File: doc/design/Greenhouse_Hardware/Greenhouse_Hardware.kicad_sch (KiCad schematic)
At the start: 4 parts, among them J1 M5Stack Watering Unit U101, J2 SSD1306 OLED Module, J3 DHT11 module, U1 ESP32-DevKitC

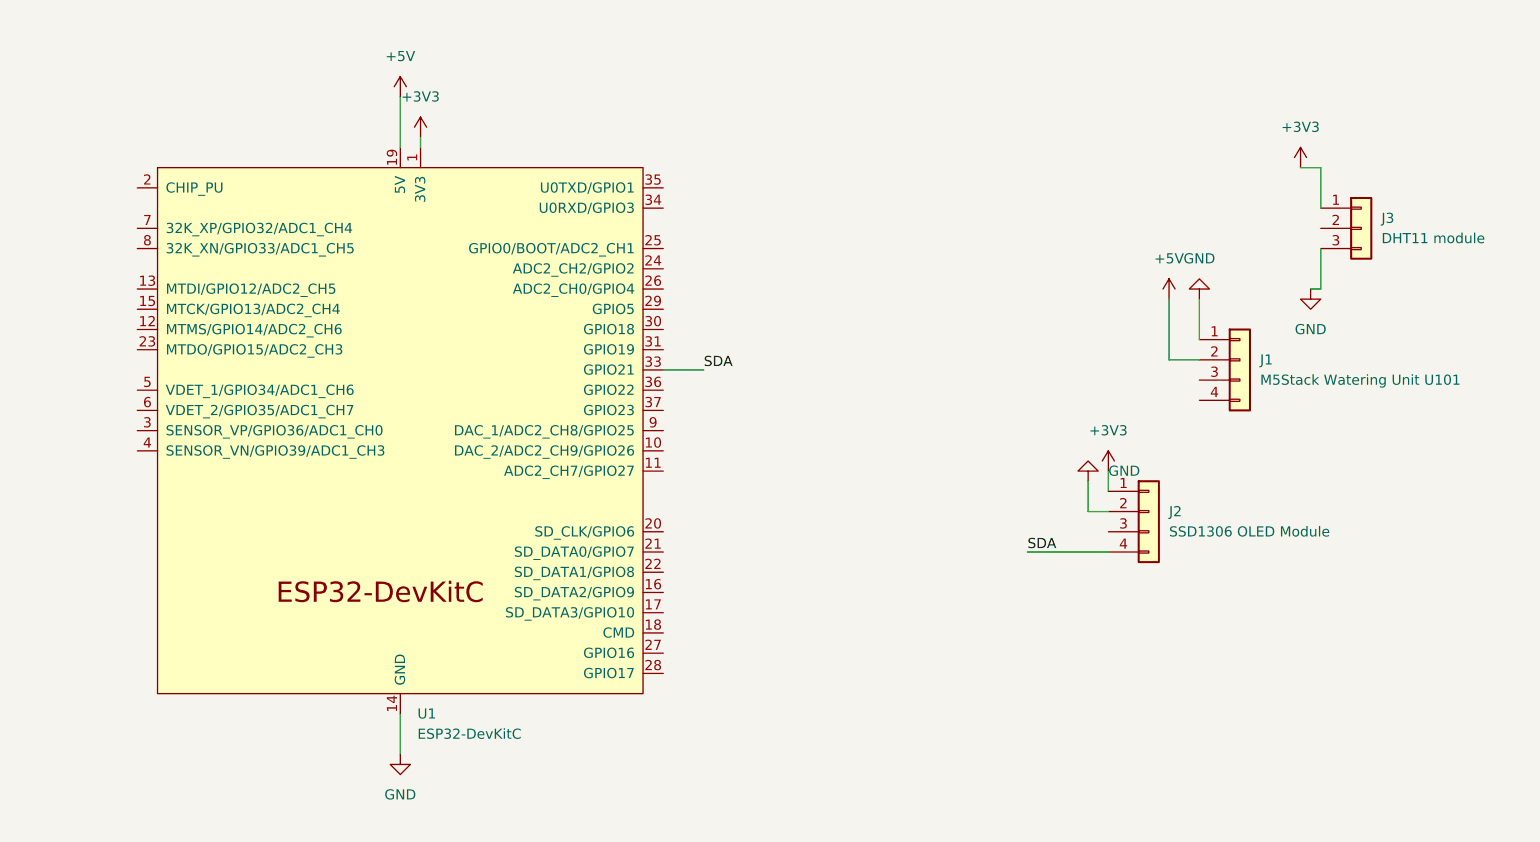
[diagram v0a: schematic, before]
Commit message: WiFi functionallity and sensor reading, validation, data display
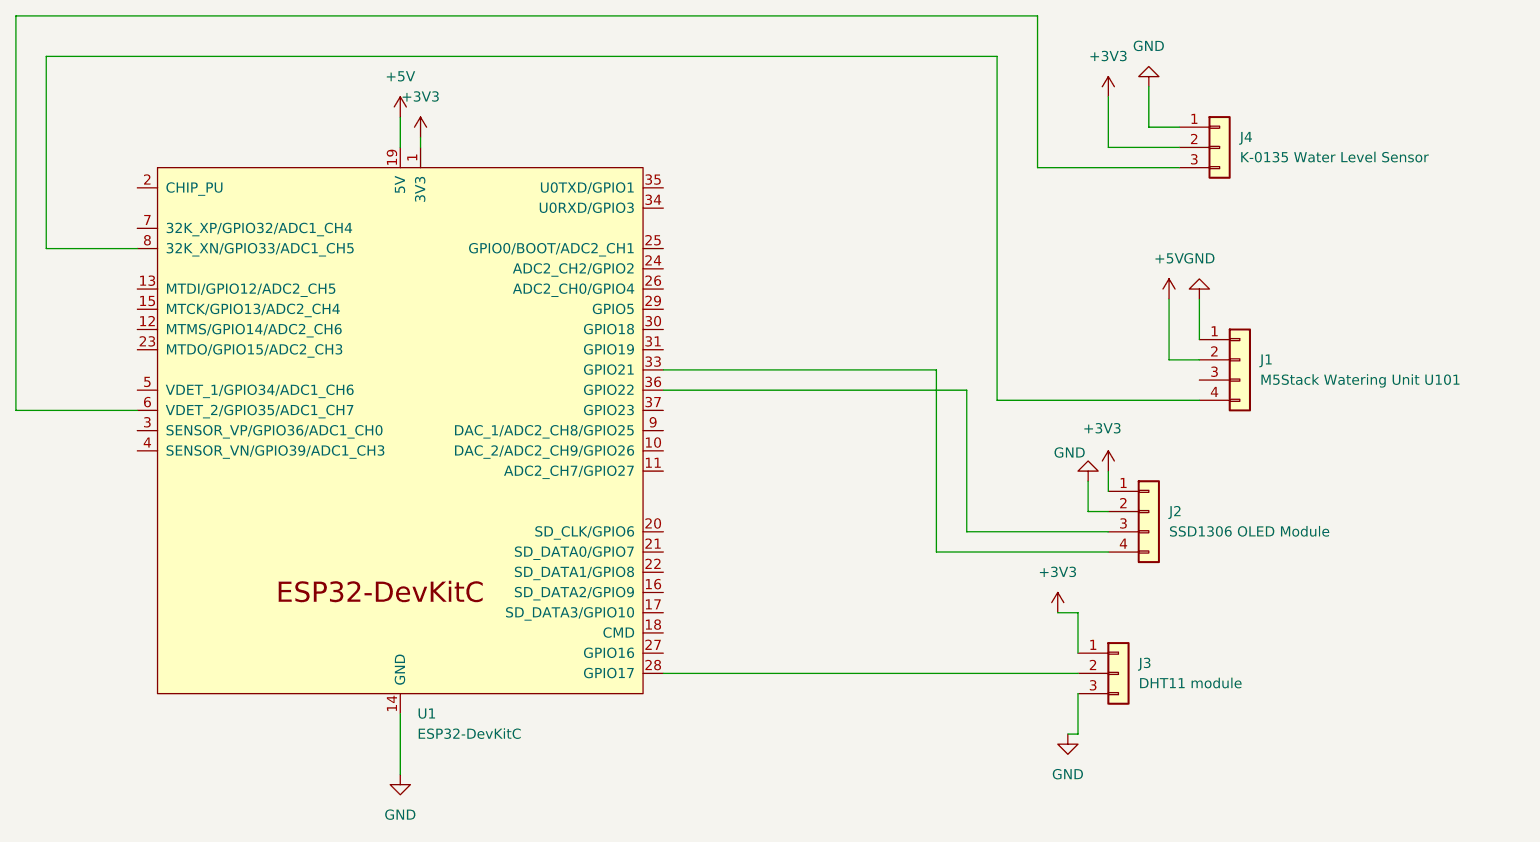
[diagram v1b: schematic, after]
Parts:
- added J4: K-0135 Water Level Sensor, symbol Connector_Generic:Conn_01x03
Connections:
- net +3V3: now also J4.2 (Pin_2)
- net GND: now also J4.1 (Pin_1)
- net at J1.4 (Pin_4): now also U1.8 (32K_XN/GPIO33/ADC1_CH5)
- net at U1.28 (GPIO17): now also J3.2 (Pin_2)
- net at U1.36 (GPIO22): now also J2.3 (Pin_3)
- net at U1.6 (VDET_2/GPIO35/ADC1_CH7): now also J4.3 (Pin_3)
- net SDA: no longer names the net of J2.4 (Pin_4), U1.33 (GPIO21)
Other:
- moved on the sheet: J3
